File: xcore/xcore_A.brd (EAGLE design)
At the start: 80 x 80 mm, 40 parts, among them U1 NC7WZ07, X1 XEF216-512-TQ128

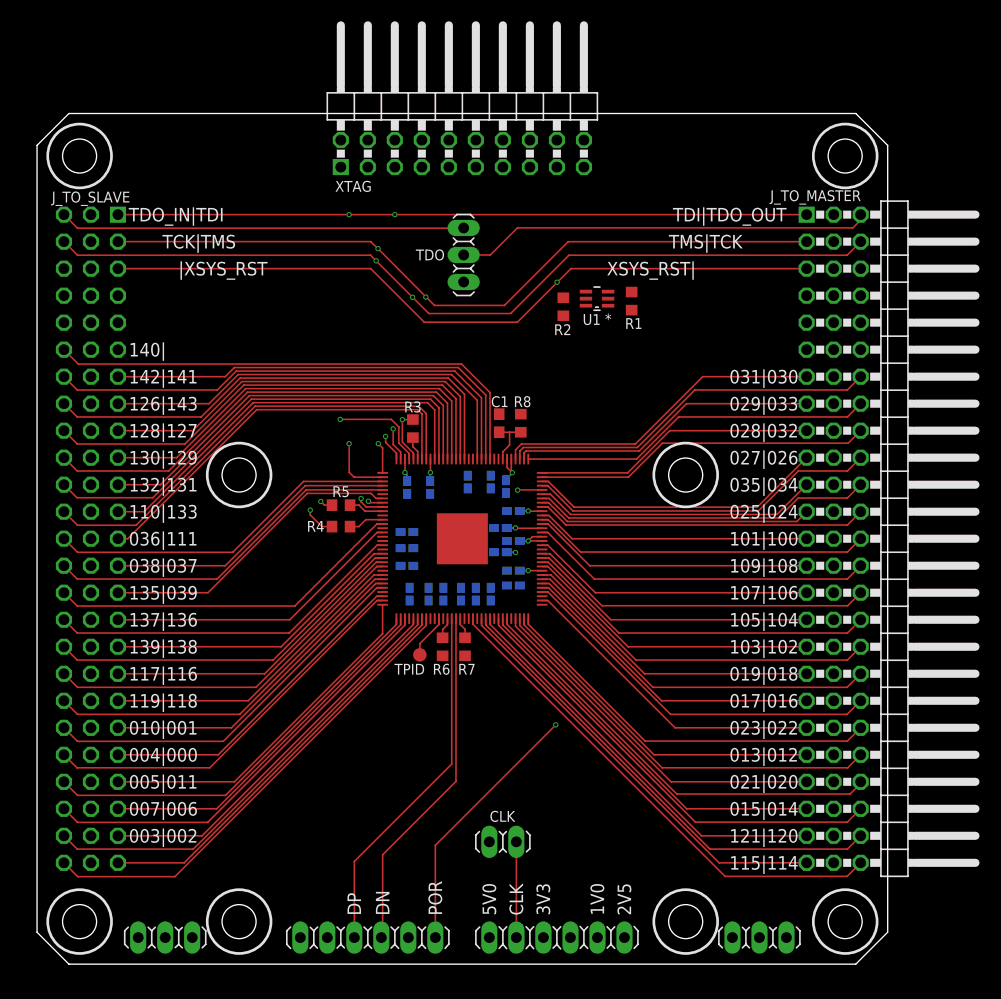
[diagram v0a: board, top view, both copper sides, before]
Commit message: xcore: WIP PCB
Signed-off-by: malo <pavol.malosek@gmail.com>
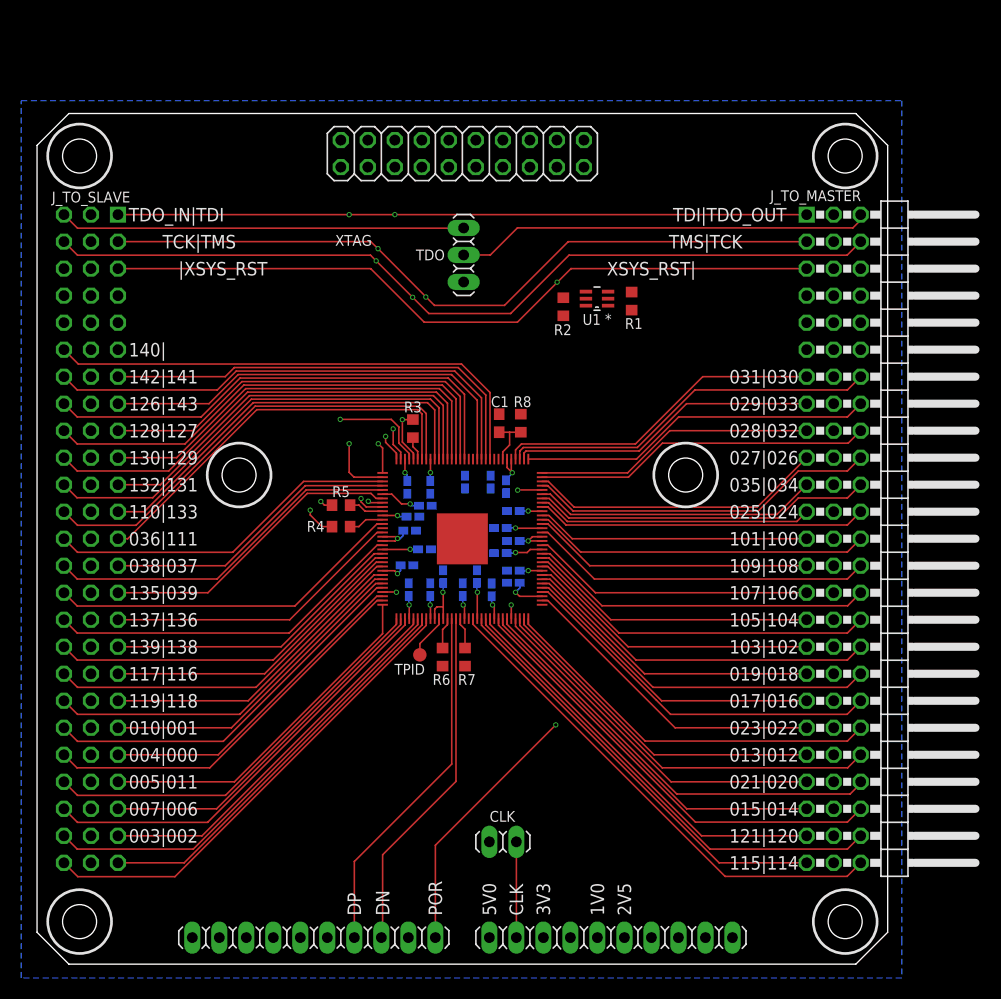
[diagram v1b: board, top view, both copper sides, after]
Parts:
- removed C24, C25, C26, C27, C28: 100n, 0603, rcl:C0402K
- removed JP1, JP2: (no value), 25pinhead:1X03
- added C31, C33, C34, C35, C36, C37, C38: 100n, 0402, rcl:C0402K
- C10, C11, C12, C13, C14, C15, C16, C17, C18, C19, C20, C21, C22, C32: value 100n, 0603 -> 100n, 0402
- XTAG: device 25pinhead:2X10/90 -> 25pinhead:2X10
- moved C22 8.01 mm to (35.4, 42.1), turned to 0 degrees
- moved XTAG 5.08 mm to (40.0, 76.2)
- moved R6 0.97 mm to (38.2, 28.9)
- moved R7 0.97 mm to (40.3, 28.9)
- moved C17 0.47 mm to (40.1, 35.2)
- moved C18 0.46 mm to (37.0, 35.2)
- moved C19 0.44 mm to (35.0, 35.2)
- moved C16 0.42 mm to (42.8, 35.2)
- moved C21 0.28 mm to (35.1, 40.8)
- moved C3 0.25 mm to (40.3, 45.3)
- moved C20 0.05 mm to (34.8, 37.5)
- renumbered C23 to C32
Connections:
- net +1V0: now also C22.2
- net +3V3: now also C31.2, C33.2, C34.2, C35.2, C36.2, C37.2, C38.2; no longer C22.2, C24.2, C25.2, C26.2, C27.2, C28.2
- net GND: now also C31.1, C33.1, C34.1, C35.1, C36.1, C37.1, C38.1; no longer C24.1, C25.1, C26.1, C27.1, C28.1
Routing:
- net +3V3: track 123.7 -> 147.1 mm, vias 3 -> 9
- net +1V0: track 60.8 -> 81.0 mm, vias 6 -> 14
- net USB_RTUNE: track 1.99 -> 2.96 mm
- net USB_VBUS: track 2.00 -> 2.96 mm
- added copper zone on layer 16, net GND

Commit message: xcore: updated with liwe 40 8x8 device
Signed-off-by: malo <pavol.malosek@gmail.com>
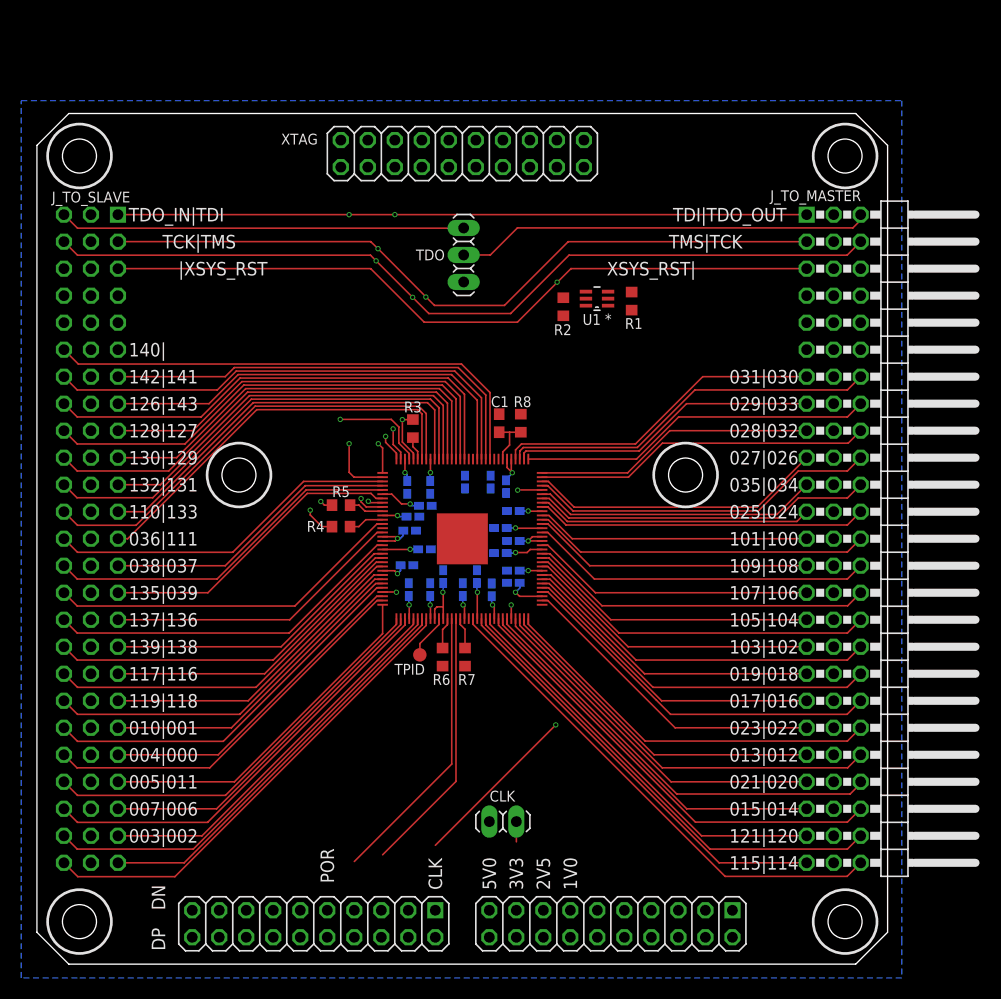
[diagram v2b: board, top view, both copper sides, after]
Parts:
- removed PWR: (no value), 25cmsquare:LIWE_12_PIN_8X8_COMPAT
- added J0: LIWE_40_PIN, 25cmsquare:LIWE_40_PIN_8X8
- moved CLK 1.90 mm to (43.8, 13.4)
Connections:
- net +1V0: now also J0.13; no longer PWR.2
- net +2V5: now also J0.15; no longer PWR.1
- net +3V3: now also J0.17; no longer PWR.4
- net +5V: now also J0.19; no longer PWR.6
- net GND: now also J0.14, J0.16, J0.18, J0.20; no longer PWR.3, PWR.8
- net IO1: now also J0.101; no longer PWR.5
- net POR: now also J0.109; no longer PWR.7
- net SCL: now also J0.105; no longer PWR.11
- net SDA: now also J0.106; no longer PWR.12
- net USB_DN: now also J0.119; no longer PWR.9
- net USB_DP: now also J0.120; no longer PWR.10
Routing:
- net +3V3: track 147.1 -> 130.9 mm
- net POR: track 59.5 -> 50.8 mm
- net USB_DN: track 32.9 -> 25.1 mm
- net USB_DP: track 33.8 -> 26.6 mm
- net IO1: track 9.00 -> 1.91 mm
- net CLK: track 54.8 -> 53.5 mm
